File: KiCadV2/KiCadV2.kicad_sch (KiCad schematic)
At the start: 39 parts, among them J1 USB_C_Receptacle_PowerOnly_6P, J2 Screw_Terminal_01x02, J3 Screw_Terminal_01x02, J4 Screw_Terminal_01x02, U1 MT3608, U2 74HC595, U3 NC7SZ157P6X, U4 NC7SZ157P6X, U5 NC7SZ157P6X, U6 74LV08AT14-13, U7 DAC082S085CISDX/NOPB, U8 MX3502S, U9 GT74LVC6G14TD

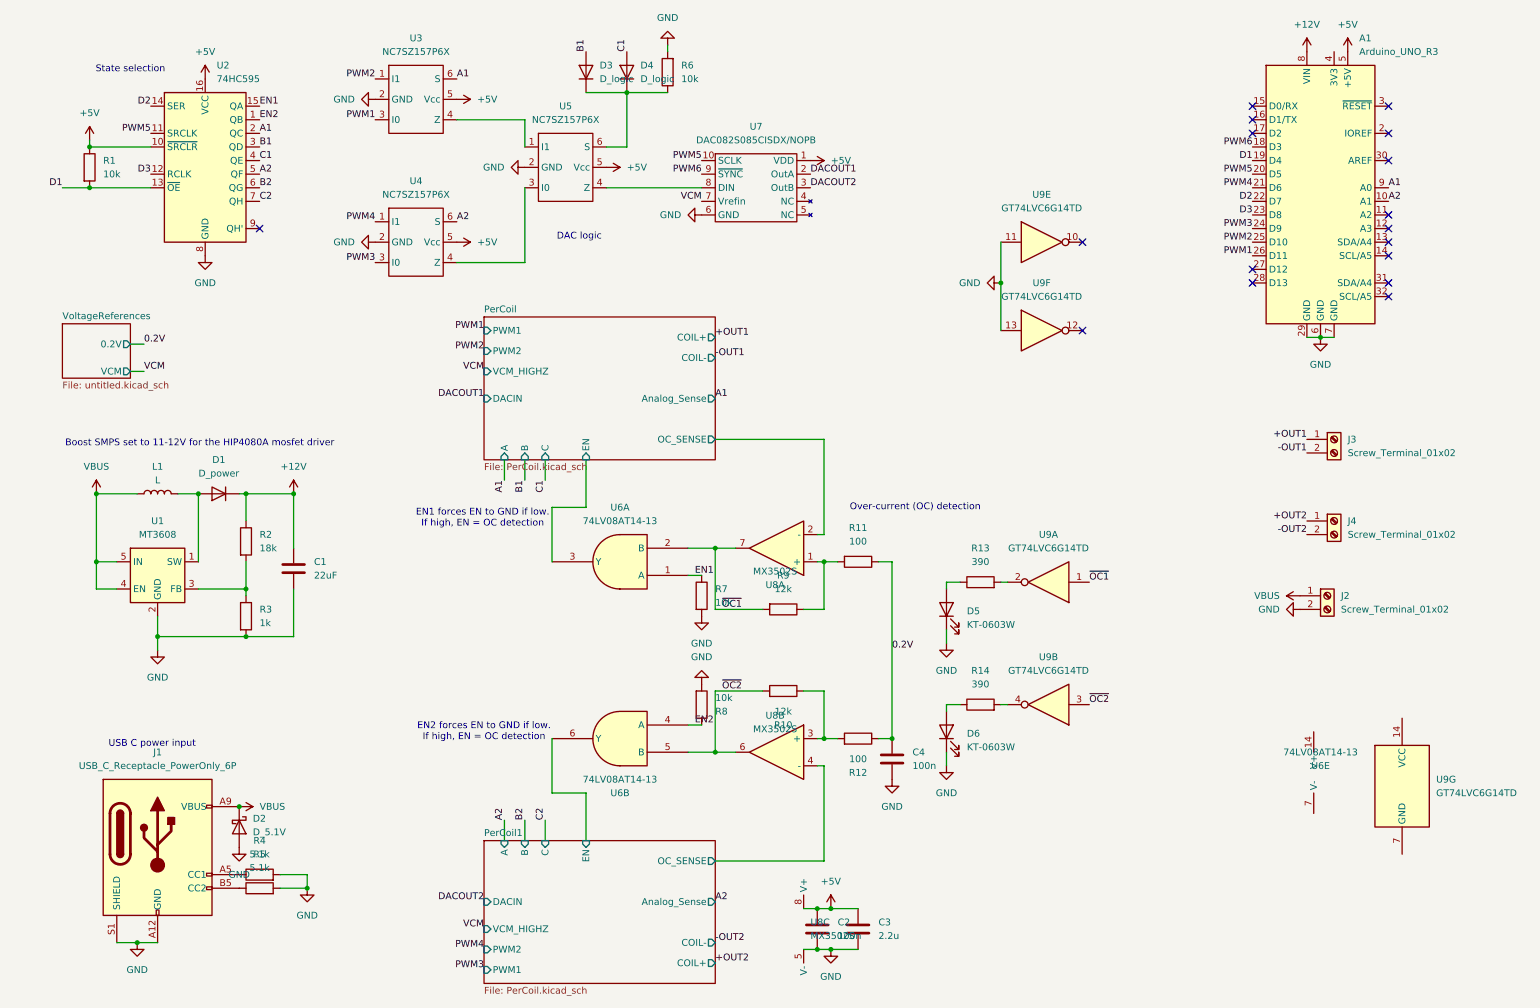
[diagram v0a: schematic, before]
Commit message: schematic FINAL! (I hope)
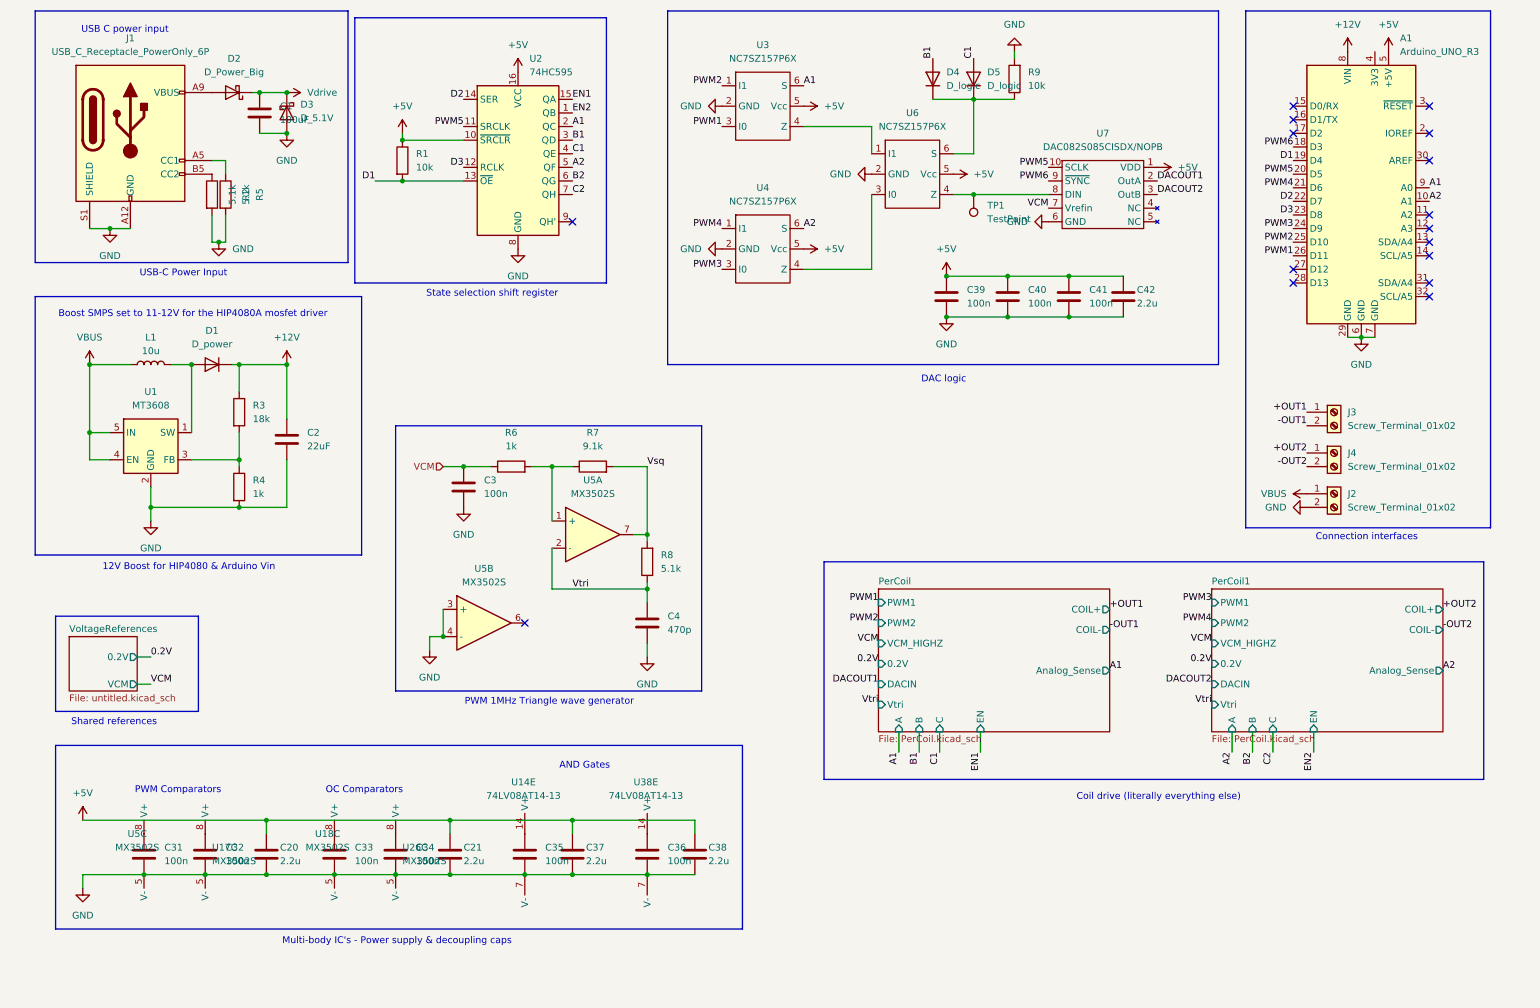
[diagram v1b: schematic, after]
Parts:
- removed C2: 100n, Capacitor_SMD:C_0603_1608Metric, symbol Device:C
- removed D5, D6: KT-0603W, LED_SMD:LED_0603_1608Metric, symbol Device:LED
- removed R10, R9: 12k, Resistor_SMD:R_0603_1608Metric, symbol Device:R
- removed R11, R12: 100, Resistor_SMD:R_0603_1608Metric, symbol Device:R
- removed R13, R14: 390, Resistor_SMD:R_0603_1608Metric, symbol Device:R
- removed U6: 74LV08AT14-13, Package_SO:TSSOP-14_4.4x5mm_P0.65mm, symbol 74xx:74LV08AT14-13
- removed U8: MX3502S, Package_SO:SOP-8_3.76x4.96mm_P1.27mm, symbol Comparator:MX3502
- removed U9: GT74LVC6G14TD, Package_SO:TSSOP-14_4.4x5mm_P0.65mm, symbol 74xx:74HC04
- added C1: 100uF, Capacitor_SMD:C_1206_3216Metric, symbol Device:C
- added C20, C21, C37, C38, C42: 2.2u, Capacitor_SMD:C_0603_1608Metric, symbol Device:C
- added C31, C32, C33, C34, C35, C36, C39, C40, C41: 100n, Capacitor_SMD:C_0603_1608Metric, symbol Device:C
- added D2: D_Power_Big, Diode_SMD:D_SMC, symbol Device:D_Schottky
- added R6: 1k, Resistor_SMD:R_0603_1608Metric, symbol Device:R
- added TP1: TestPoint, TestPoint:TestPoint_Pad_D2.5mm, symbol Connector:TestPoint
- added U14, U38: 74LV08AT14-13, Package_SO:TSSOP-14_4.4x5mm_P0.65mm, symbol 74xx:74LV08AT14-13
- added U17, U18, U26, U5: MX3502S, Package_SO:SOP-8_3.76x4.96mm_P1.27mm, symbol Comparator:MX3502
- C3: value 2.2u -> 100n; LCSC C23630 -> C14663
- C4: value 100n -> 470p; LCSC C14663 -> C396711
- D3: renamed from D2; footprint Diode_SMD:D_SMA -> Diode_SMD:D_SMB; LCSC (none) -> C19077494
- L1: value L -> 10u; footprint (none) -> Inductor_SMD:10uH C15029
- R7: value 10k -> 9.1k; LCSC C25804 -> C23260
- R8: value 10k -> 5.1k; LCSC C25804 -> C23186
- renumbered C1 to C2, D3 to D4, D4 to D5, R5 to R2, R2 to R3, R3 to R4, R4 to R5, R6 to R9, U5 to U6
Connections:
- net +5V: now also C20.1, C21.1, C37.1, C38.1, C39.1, C40.1, C41.1, C42.1; no longer C3.2
- net 0.2V: no longer C4.2
- net EN1: no longer R7.1
- net EN2: no longer R8.1
- net GND: now also C3.2, C4.2, C1.2, C20.2, C21.2, C31.2, C32.2, C33.2, C34.2, C35.2, C36.2, C37.2, C38.2, C39.2, C40.2, C41.2, C42.2, U14.7 (V-), U17.5 (V-), U18.5 (V-), U26.5 (V-), U38.7 (V-), U5.3 (+), U5.4 (-), U5.5 (V-); no longer C3.1, C4.1, R7.2, R8.2
- net VBUS: no longer D3.1 (K), J1.A9 (VBUS), J1.B9 (VBUS)
- net VCM: now also C3.1, R6.1
- net at U6.4 (Z), U7.8 (DIN): now also TP1.1
- new net: C32.1, U17.8 (V+)
- new net: C35.1, U14.14 (V+)
- new net: C36.1, U38.14 (V+)
- new net: C31.1, U5.8 (V+)
- new net: R6.2, R7.1, U5.1 (+)
- new net: D2.2 (A), J1.A9 (VBUS), J1.B9 (VBUS)
- new net: C34.1, U26.8 (V+)
- new net: C33.1, U18.8 (V+)
- new net Vdrive: C1.1, D2.1 (K), D3.1 (K)
- new net Vsq: R7.2, R8.2, U5.7
- new net Vtri: C4.1, R8.1, U5.2 (-)
- no-connect marks 17 -> 16
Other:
- sheet PerCoil ports: added 0.2V, Vtri; removed OC_SENSE
- sheet PerCoil1 ports: added 0.2V, Vtri; removed OC_SENSE
- note added: "12V Boost for HIP4080 & Arduino Vin"
- note added: "AND Gates"
- note added: "Coil drive (literally everything else)"
- note added: "Connection interfaces"
- note added: "Multi-body IC's - Power supply & decoupling caps"
- note added: "OC Comparators"
- note added: "PWM 1MHz Triangle wave generator"
- note added: "PWM Comparators"
- note added: "Shared references"
- note added: "State selection shift register"
- note added: "USB-C Power Input"
- note removed: "EN1 forces EN to GND if low. If high, EN = OC detection"
- note removed: "EN2 forces EN to GND if low. If high, EN = OC detection"
- note removed: "Over-current (OC) detection"
- note removed: "State selection"
- moved on the sheet: A1, C2, D1, D3, D4, D5, J1, J2, J3, J4, L1, R1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
